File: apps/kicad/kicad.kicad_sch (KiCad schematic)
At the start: 10 parts, among them J1 XMC4200 DE-9 (used pins), U1 XMC4200 (used pins), U2 LCD 16x2, U3 AHT10, U4 GPS NEO-6M, U5 POTENTIOMETER, U6 EEPROM, U7 CAN USB TRANSCEIVER

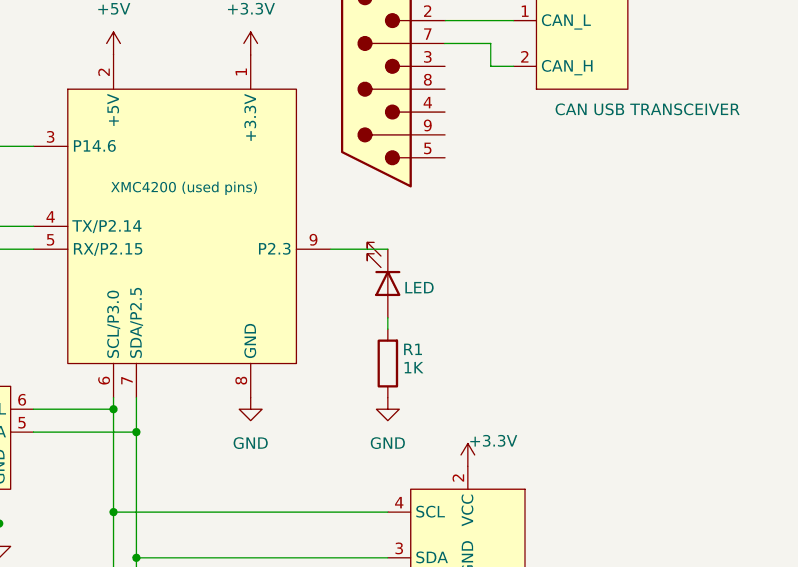
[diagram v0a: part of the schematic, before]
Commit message: schematic change, reflect dependent files
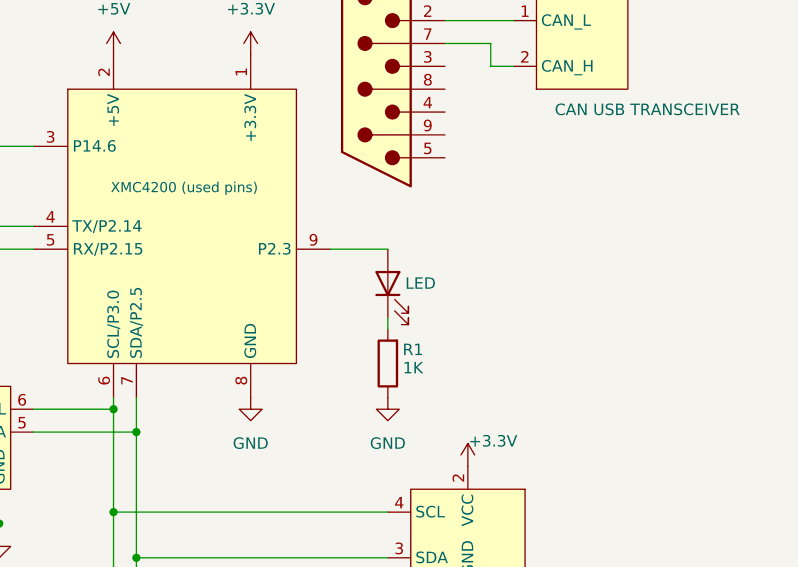
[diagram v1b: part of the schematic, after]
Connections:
- net at R1.2: now also D1.1 (K); no longer D1.2 (A)
- net at U1.9 (P2.3): now also D1.2 (A); no longer D1.1 (K)
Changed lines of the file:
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@@
 	(symbol
 		(lib_id "Device:LED")
-		(at 132.08 106.68 270)
+		(at 132.08 106.68 90)
 		(unit 1)
 		(body_style 1)
@@
 		(dnp no)
 		(property "Reference" "D1"
-			(at 138.43 105.0925 0)
+			(at 125.73 108.2675 0)
 			(hide yes)
 			(show_name no)
@@
 		)
 		(property "Value" "LED"
-			(at 133.858 107.188 90)
+			(at 137.414 106.68 90)
 			(show_name no)
 			(do_not_autoplace no)
